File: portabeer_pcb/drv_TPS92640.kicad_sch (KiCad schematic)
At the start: 23 parts, among them Q12 Si7336ADP, Q16 Si7336ADP, U14 TPS92640PWP/NOPB

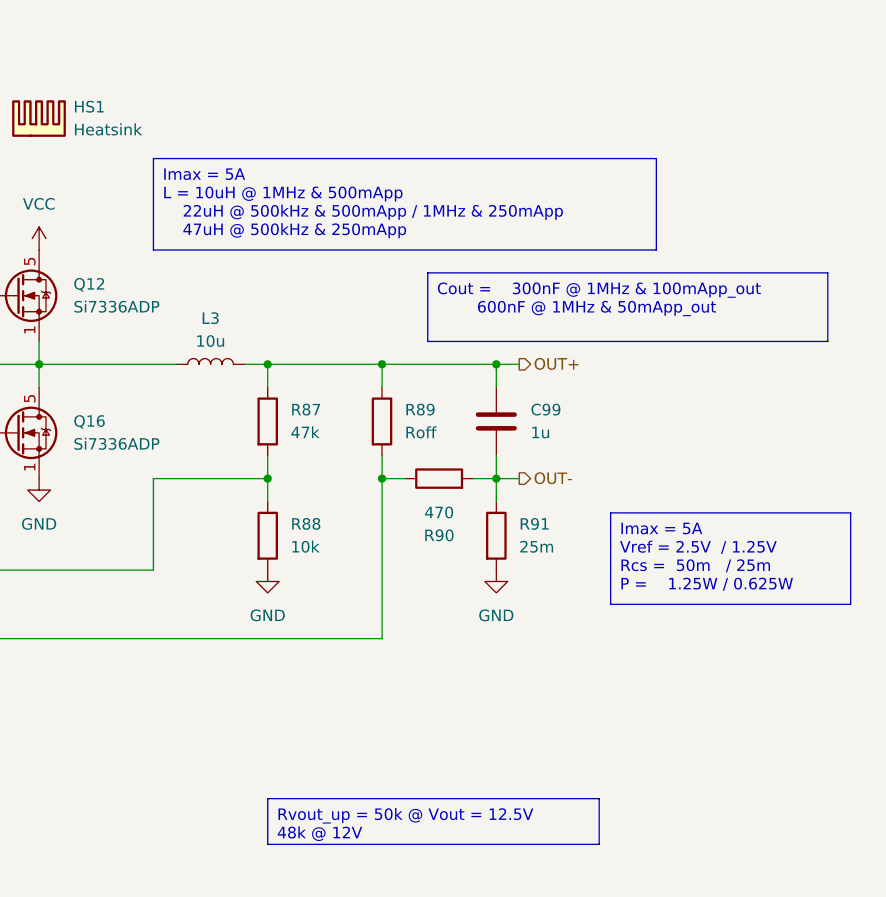
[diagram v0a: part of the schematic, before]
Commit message: partial routing
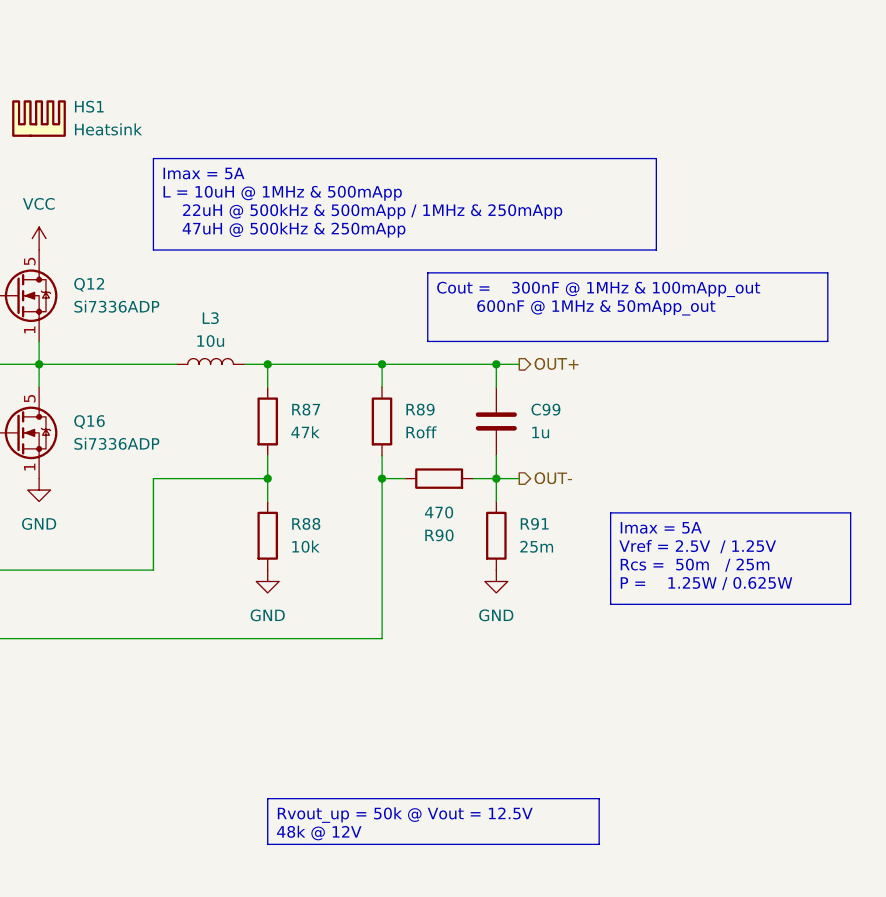
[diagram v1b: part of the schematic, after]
